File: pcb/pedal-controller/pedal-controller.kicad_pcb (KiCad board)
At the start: 2 copper layers, 57.1 x 76.2 mm, 9 parts

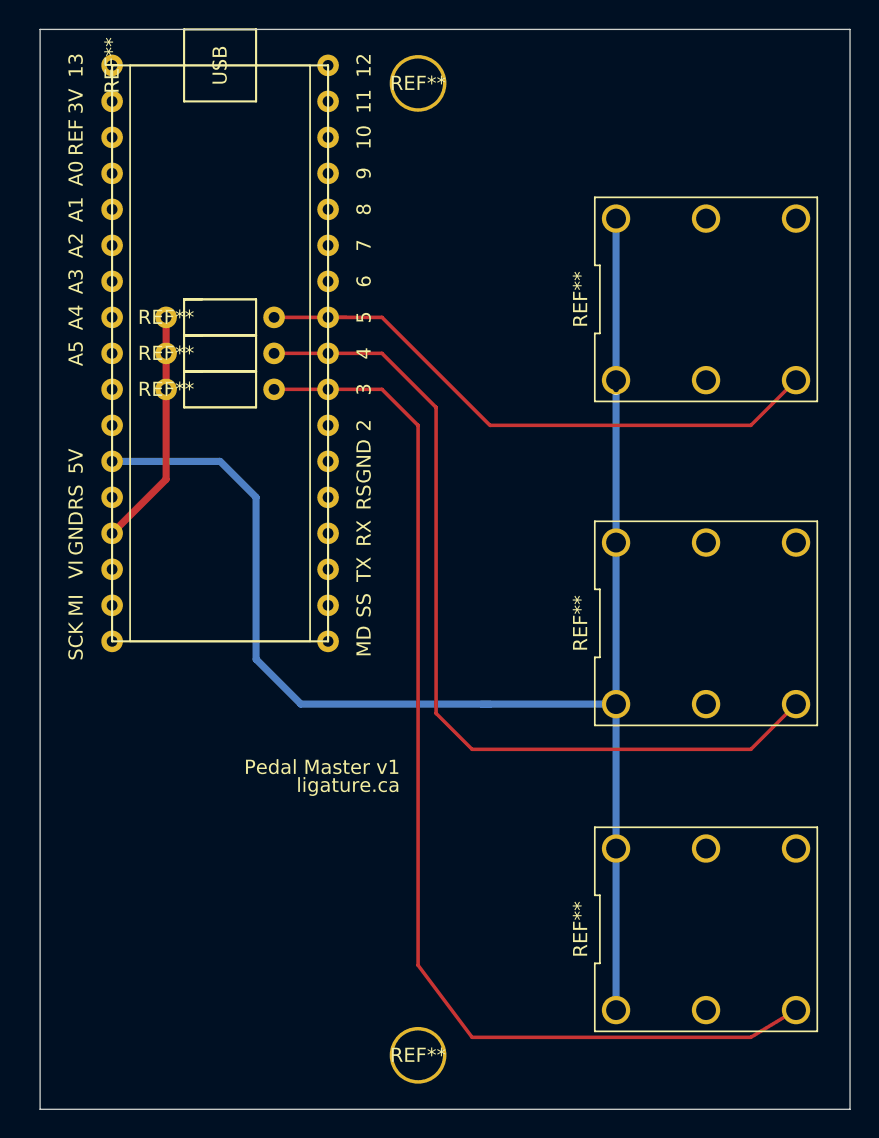
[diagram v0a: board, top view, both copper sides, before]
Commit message: ordered version 3
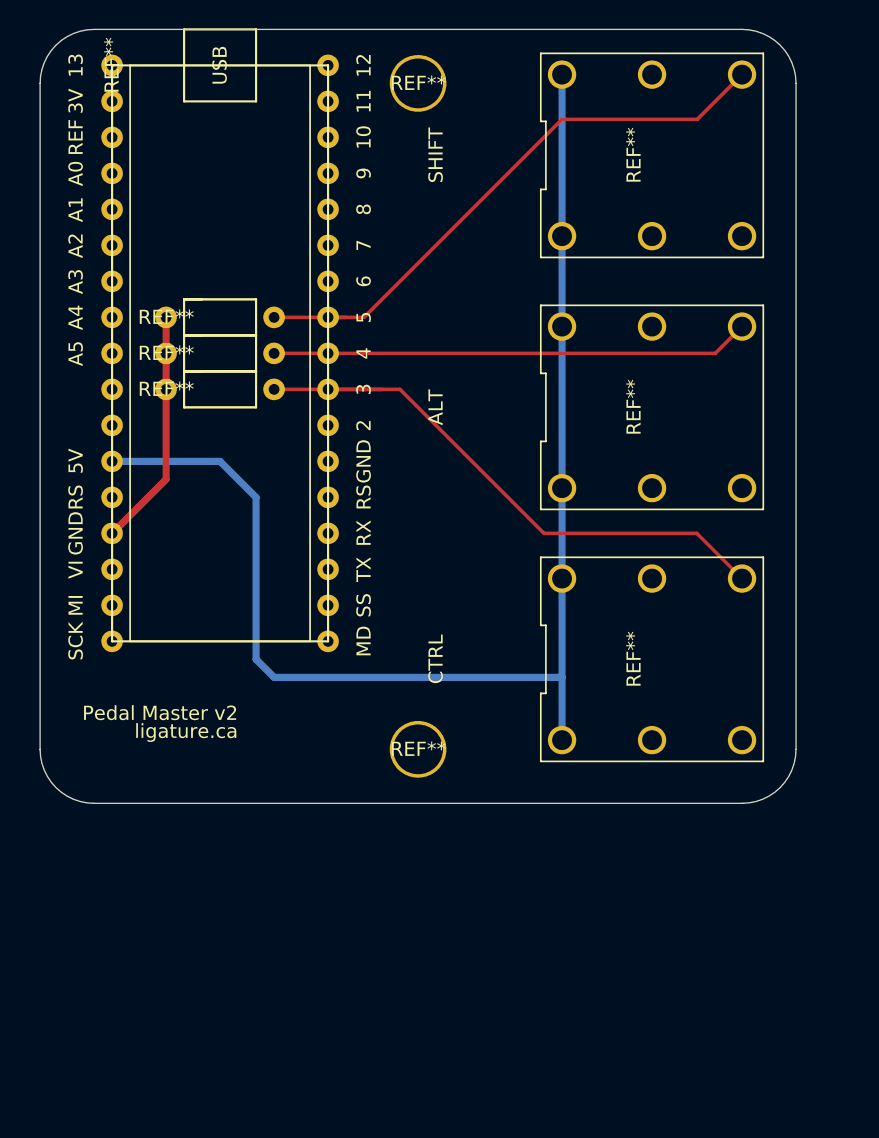
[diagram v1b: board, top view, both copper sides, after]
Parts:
- moved REF** 21.6 mm to (144.8, 106.7)
- moved REF** 19.4 mm to (161.3, 100.3)
- moved REF** 15.7 mm to (161.3, 82.5)
- moved REF** 10.9 mm to (161.3, 64.8)
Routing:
- net (no net): track 307.3 -> 226.7 mm, vias 1 -> 0
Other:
- board size 57.1 x 76.2 mm -> 53.3 x 54.6 mm
- board text added: "ALT"
- board text added: "CTRL"
- board text added: "Pedal Master v2"
- board text added: "SHIFT"
- board text removed: "Pedal Master v1"
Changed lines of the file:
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@@
   (general
     (thickness 1.6)
-    (drawings 21)
-    (tracks 34)
+    (drawings 28)
+    (tracks 26)
     (zones 0)
     (modules 9)
@@
   )
   (module pedal-controller:mounting-hole (layer F.Cu)
-    (at 144.78 128.27)
+    (at 144.78 106.68)
     (fp_text reference REF** (at 0 0) (layer F.SilkS)
       (effects (font (size 1 1) (thickness 0.15)))
@@
   )
   (module pedal-controller:ACJS-MHDR_Jack_Connector (layer F.Cu)
-    (at 165.1 119.38)
-    (fp_text reference REF** (at -8.85 0 90) (layer F.SilkS)
+    (at 161.29 100.33)
+    (fp_text reference REF** (at -1.27 0 90) (layer F.SilkS)
       (effects (font (size 1 1) (thickness 0.15)))
     )
@@
   )
   (module pedal-controller:ACJS-MHDR_Jack_Connector (layer F.Cu)
-    (at 165.1 97.79)
-    (fp_text reference REF** (at -8.85 0 90) (layer F.SilkS)
+    (at 161.29 82.55)
+    (fp_text reference REF** (at -1.27 0 90) (layer F.SilkS)
       (effects (font (size 1 1) (thickness 0.15)))
     )
@@
   )
   (module pedal-controller:ACJS-MHDR_Jack_Connector (layer F.Cu)
-    (at 165.1 74.93)
-    (fp_text reference REF** (at -8.85 0 90) (layer F.SilkS)
+    (at 161.29 64.77)
+    (fp_text reference REF** (at -1.27 0 90) (layer F.SilkS)
       (effects (font (size 1 1) (thickness 0.15)))
     )
@@
     (pad 6 thru_hole circle (at -6.35 -5.7) (size 2 2) (drill 1.4) (layers *.Cu *.Mask))
   )
-  (gr_line (start 118.11 132.08) (end 118.11 55.88) (layer Edge.Cuts) (width 0.05))
-  (gr_line (start 175.26 132.08) (end 118.11 132.08) (layer Edge.Cuts) (width 0.05))
-  (gr_line (start 175.26 55.88) (end 175.26 132.08) (layer Edge.Cuts) (width 0.05))
-  (gr_line (start 118.11 55.88) (end 175.26 55.88) (layer Edge.Cuts) (width 0.05))
-  (gr_text "Pedal Master v1" (at 143.51 107.95) (layer F.SilkS)
+  (gr_text SHIFT (at 146.05 64.77 90) (layer F.SilkS)
+    (effects (font (size 1 1) (thickness 0.15)))
+  )
+  (gr_text ALT (at 146.05 82.55 90) (layer F.SilkS)
+    (effects (font (size 1 1) (thickness 0.15)))
+  )
+  (gr_text CTRL (at 146.05 100.33 90) (layer F.SilkS)
+    (effects (font (size 1 1) (thickness 0.15)))
+  )
+  (gr_line (start 167.64 55.88) (end 121.92 55.88) (layer Edge.Cuts) (width 0.05))
+  (gr_line (start 171.45 106.68) (end 171.45 59.69) (layer Edge.Cuts) (width 0.05))
+  (gr_line (start 121.92 110.49) (end 167.64 110.49) (layer Edge.Cuts) (width 0.05))
+  (gr_line (start 118.11 59.69) (end 118.11 106.68) (layer Edge.Cuts) (width 0.05))
+  (gr_arc (start 121.92 59.69) (end 121.92 55.88) (angle -90) (layer Edge.Cuts) (width 0.05))
+  (gr_arc (start 121.92 106.68) (end 118.11 106.68) (angle -90) (layer Edge.Cuts) (width 0.05))
+  (gr_arc (start 167.64 106.68) (end 167.64 110.49) (angle -90) (layer Edge.Cuts) (width 0.05))
+  (gr_arc (start 167.64 59.69) (end 171.45 59.69) (angle -90) (layer Edge.Cuts) (width 0.05))
+  (gr_text "Pedal Master v2" (at 132.08 104.14) (layer F.SilkS)
     (effects (font (size 1 1) (thickness 0.15)) (justify right))
   )
-  (gr_text ligature.ca (at 143.51 109.22) (layer F.SilkS)
+  (gr_text ligature.ca (at 132.08 105.41) (layer F.SilkS)
     (effects (font (size 1 1) (thickness 0.15)) (justify right))
   )
@@
   (gr_line (start 133.35 74.93) (end 133.35 77.47) (layer F.SilkS) (width 0.12))
   (gr_line (start 128.27 74.93) (end 133.35 74.93) (layer F.SilkS) (width 0.12))
-  (segment (start 158.75 103.49) (end 158.75 113.68) (width 0.5) (layer B.Cu) (net 0) (status 30))
   (segment (start 138.43 76.2) (end 134.62 76.2) (width 0.25) (layer F.Cu) (net 0) (status 30))
   (segment (start 138.43 78.74) (end 134.62 78.74) (width 0.25) (layer F.Cu) (net 0) (status 30))
   (segment (start 138.43 81.28) (end 134.62 81.28) (width 0.25) (layer F.Cu) (net 0) (status 30))
-  (segment (start 158.75 81.28) (end 158.75 80.63) (width 0.25) (layer B.Cu) (net 0) (status 30))
-  (segment (start 158.75 113.68) (end 158.75 125.08) (width 0.5) (layer B.Cu) (net 0) (status 30))
-  (segment (start 158.75 103.49) (end 158.75 69.23) (width 0.5) (layer B.Cu) (net 0) (status 30))
+  (segment (start 154.94 71.12) (end 154.94 70.47) (width 0.25) (layer B.Cu) (net 0) (status 30))
   (segment (start 130.81 86.36) (end 133.35 88.9) (width 0.5) (layer B.Cu) (net 0))
   (segment (start 123.19 86.36) (end 130.81 86.36) (width 0.5) (layer B.Cu) (net 0) (status 10))
   (segment (start 133.35 88.9) (end 133.35 100.33) (width 0.5) (layer B.Cu) (net 0))
-  (segment (start 133.35 100.33) (end 136.51 103.49) (width 0.5) (layer B.Cu) (net 0))
-  (segment (start 136.51 103.49) (end 149.86 103.49) (width 0.5) (layer B.Cu) (net 0))
   (segment (start 127 76.2) (end 127 87.63) (width 0.5) (layer F.Cu) (net 0) (status 10))
   (segment (start 127 87.63) (end 123.19 91.44) (width 0.5) (layer F.Cu) (net 0) (status 20))
-  (segment (start 149.86 83.82) (end 168.26 83.82) (width 0.25) (layer F.Cu) (net 0))
-  (segment (start 168.26 83.82) (end 171.45 80.63) (width 0.25) (layer F.Cu) (net 0) (status 20))
-  (segment (start 142.24 76.2) (end 149.86 83.82) (width 0.25) (layer F.Cu) (net 0))
-  (segment (start 138.43 76.2) (end 142.24 76.2) (width 0.25) (layer F.Cu) (net 0) (status 10))
-  (segment (start 148.59 106.68) (end 168.26 106.68) (width 0.25) (layer F.Cu) (net 0))
-  (segment (start 168.26 106.68) (end 171.45 103.49) (width 0.25) (layer F.Cu) (net 0) (status 20))
-  (segment (start 146.05 104.14) (end 148.59 106.68) (width 0.25) (layer F.Cu) (net 0))
-  (segment (start 146.05 82.55) (end 146.05 104.14) (width 0.25) (layer F.Cu) (net 0))
-  (segment (start 142.24 78.74) (end 146.05 82.55) (width 0.25) (layer F.Cu) (net 0))
-  (segment (start 138.43 78.74) (end 142.24 78.74) (width 0.25) (layer F.Cu) (net 0) (status 10))
-  (segment (start 149.24 103.49) (end 158.75 103.49) (width 0.5) (layer B.Cu) (net 0) (status 20))
   (segment (start 139.7 76.2) (end 138.43 76.2) (width 0.25) (layer F.Cu) (net 0) (status 20))
   (segment (start 138.43 81.28) (end 138.43 81.28) (width 0.25) (layer F.Cu) (net 0))
-  (via (at 158.75 81.28) (size 0.8) (drill 0.4) (layers F.Cu B.Cu) (net 0))
-  (segment (start 168.26 127) (end 171.45 125.08) (width 0.25) (layer F.Cu) (net 0))
-  (segment (start 144.78 121.92) (end 148.59 127) (width 0.25) (layer F.Cu) (net 0))
-  (segment (start 144.78 83.82) (end 144.78 121.92) (width 0.25) (layer F.Cu) (net 0))
-  (segment (start 148.59 127) (end 168.26 127) (width 0.25) (layer F.Cu) (net 0))
   (segment (start 138.43 81.28) (end 142.24 81.28) (width 0.25) (layer F.Cu) (net 0))
-  (segment (start 142.24 81.28) (end 144.78 83.82) (width 0.25) (layer F.Cu) (net 0))
+  (segment (start 138.43 76.2) (end 140.97 76.2) (width 0.25) (layer F.Cu) (net 0))
+  (segment (start 140.97 76.2) (end 154.94 62.23) (width 0.25) (layer F.Cu) (net 0))
+  (segment (start 138.43 81.28) (end 143.51 81.28) (width 0.25) (layer F.Cu) (net 0))
+  (segment (start 143.51 81.28) (end 153.67 91.44) (width 0.25) (layer F.Cu) (net 0))
+  (segment (start 164.45 91.44) (end 167.64 94.63) (width 0.25) (layer F.Cu) (net 0))
+  (segment (start 133.35 100.33) (end 134.62 101.6) (width 0.5) (layer B.Cu) (net 0))
+  (segment (start 154.94 106.03) (end 154.94 101.6) (width 0.5) (layer B.Cu) (net 0))
+  (segment (start 154.94 101.6) (end 154.94 59.07) (width 0.5) (layer B.Cu) (net 0))
+  (segment (start 164.48 62.23) (end 167.64 59.07) (width 0.25) (layer F.Cu) (net 0))
+  (segment (start 154.94 62.23) (end 164.48 62.23) (width 0.25) (layer F.Cu) (net 0))
+  (segment (start 165.75 78.74) (end 167.64 76.85) (width 0.25) (layer F.Cu) (net 0))
+  (segment (start 138.43 78.74) (end 165.75 78.74) (width 0.25) (layer F.Cu) (net 0))
+  (segment (start 153.67 91.44) (end 164.45 91.44) (width 0.25) (layer F.Cu) (net 0))
+  (segment (start 134.62 101.6) (end 154.94 101.6) (width 0.5) (layer B.Cu) (net 0))
 )
